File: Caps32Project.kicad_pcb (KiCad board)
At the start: 2 copper layers, 20.8 x 24.6 mm, 53 parts, among them J1 USB_C_Receptacle_USB2.0_16P, J2 SH1.0, Q1 AO3401A, SW1 Reset, SW2 Boot, SW3 SW_SPDT, U1 MPU-6050, U2 AP2112K-3.3, U3 MCP73831-2-OT, U4 ESP32-S2, Y1 40MHz

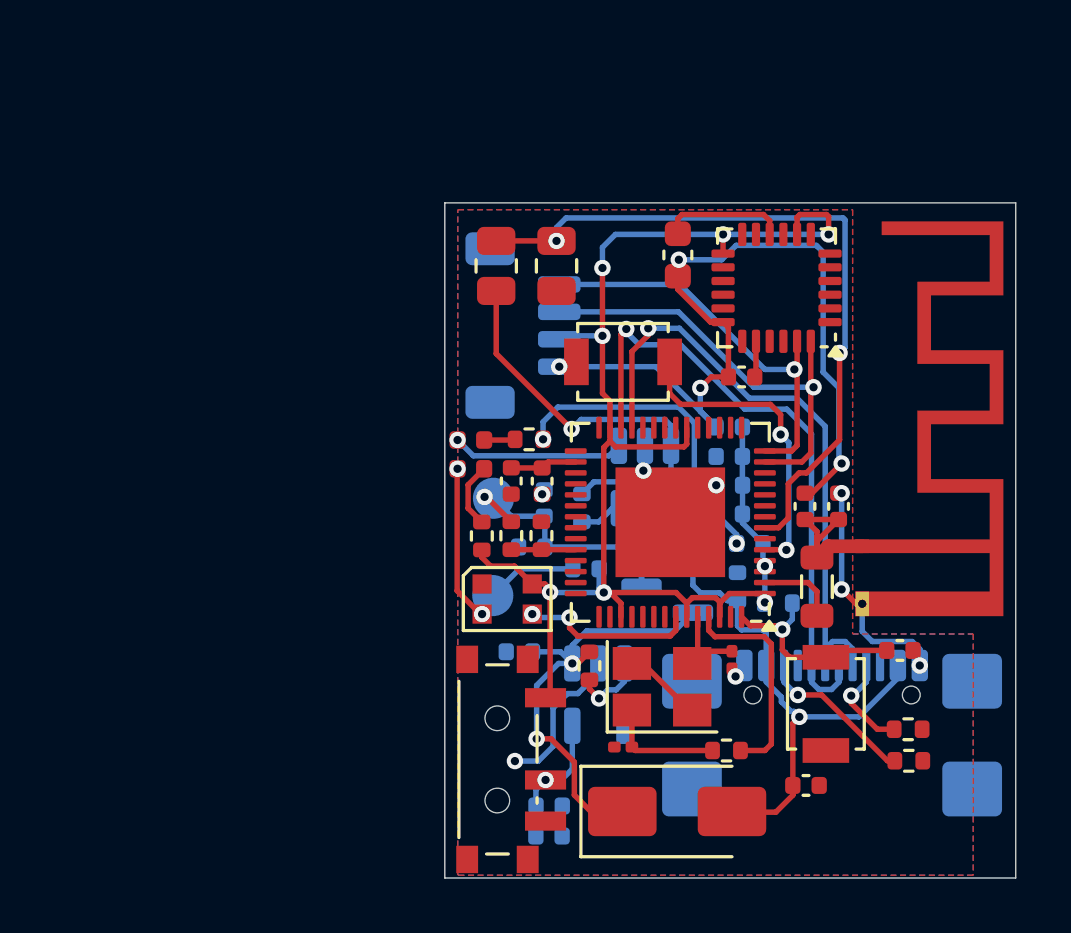
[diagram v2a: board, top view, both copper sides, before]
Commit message: Update Board
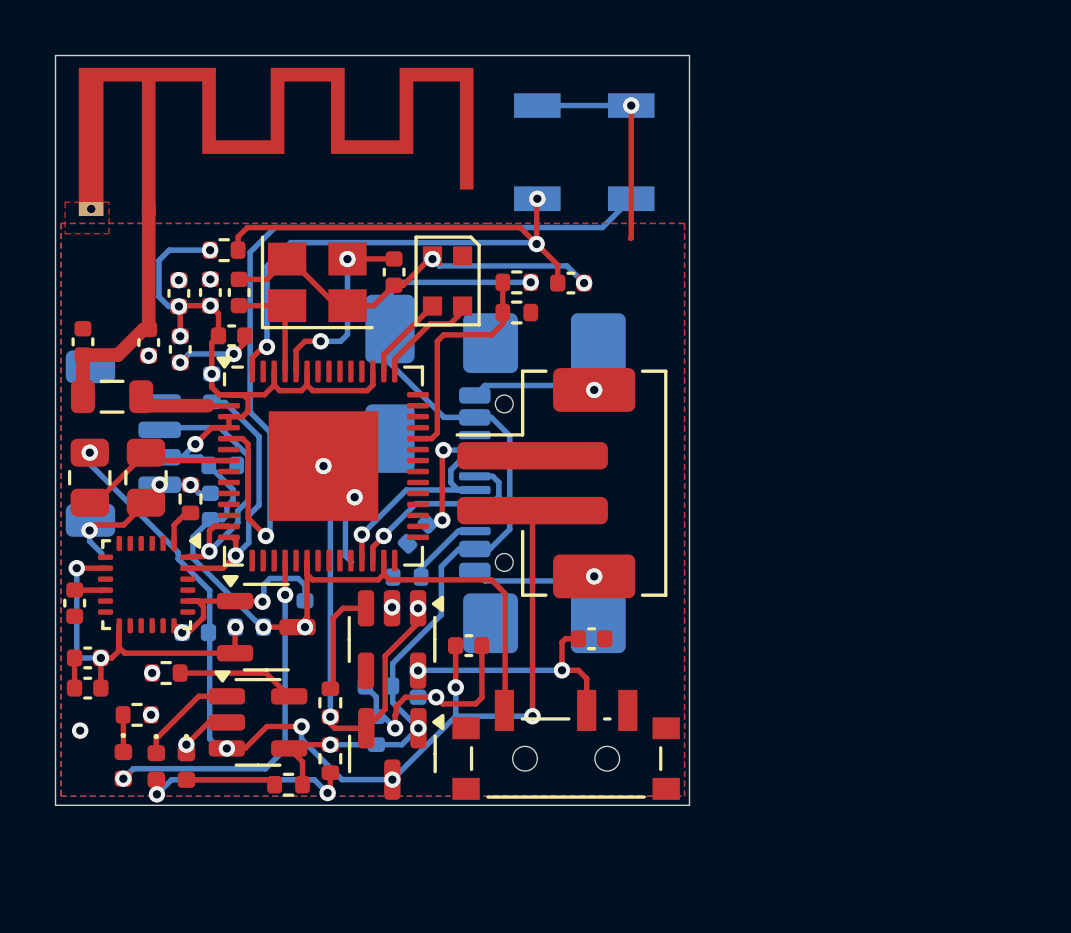
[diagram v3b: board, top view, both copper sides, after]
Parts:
- removed TP1, TP2: TestPoint, TestPoint:TestPoint_Pad_D1.5mm
- added C22: 0.1uF, Capacitor_SMD:C_0402_1005Metric, F.Cu at (112.4, 49.1)
- added C23: 1uF, Capacitor_SMD:C_0402_1005Metric, F.Cu at (110.0, 49.0)
- added D5: WS2812B, LED_SMD:LED_WS2812B-2020_PLCC4_2.0x2.0mm, F.Cu at (123.3, 46.8)
- added J3: USB_C_Receptacle_USB2.0_16P, Connector_USB:USB_C_Receptacle_GCT_USB4110, B.Cu at (128.0, 54.2)
- added R14: 2K, Resistor_SMD:R_0402_1005Metric, F.Cu at (125.8, 48.0)
- added R15: 2K, Resistor_SMD:R_0402_1005Metric, F.Cu at (113.1, 61.1)
- added R16: 5.1K, Resistor_SMD:R_0402_1005Metric, B.Cu at (122.2, 56.0)
- added R17: 5.1K, Resistor_SMD:R_0402_1005Metric, B.Cu at (121.8, 57.6)
- added U5: ESP32-S2, Package_DFN_QFN:QFN-56-1EP_7x7mm_P0.4mm_EP4x4mm, F.Cu at (118.8, 53.6)
- AE1: footprint RF_Antenna:Texas_SWRA117D_2.4GHz_Left -> RF_Antenna:Texas_SWRA117D_2.4GHz_Right
- C1: value 1.0uF -> 1uF; moved to F.Cu
- C10: value 15pF -> 0.1uF; footprint Capacitor_SMD:C_0201_0603Metric -> Capacitor_SMD:C_0402_1005Metric; moved to B.Cu
- C11: value 4.7uF -> 1.0uF; moved to F.Cu
- C12: value 1.0uF -> 0.1uF
- C13, C19: value 0.1uF -> 10uF
- C14: value 1uF -> 0.1uF; moved to F.Cu
- C16, C18, Q1, R8, R9, U2: moved to F.Cu
- C17: value 0.1uF -> 1uF; moved to F.Cu
- C2: value 0.1uF -> 1uF
- C20, C21: value 1uF -> 15pF
- C3: value 1uF -> 1.0uF; moved to B.Cu
- C5: value 1.0uF -> 0.1uF; moved to F.Cu
- C6: value 2.2nF -> 1uF; footprint Capacitor_SMD:C_0603_1608Metric -> Capacitor_SMD:C_0402_1005Metric
- C7, D2: moved to B.Cu
- C8: value 4.7uF -> 1uF; moved to B.Cu
- C9: value 15pF -> 1.0uF; footprint Capacitor_SMD:C_0201_0603Metric -> Capacitor_SMD:C_0402_1005Metric; moved to B.Cu
- D1: value LED -> RED
- D3: value LED -> BLUE
- D4: value WS2812B-2020 -> Orange; footprint LED_SMD:LED_WS2812B-2020_PLCC4_2.0x2.0mm -> LED_SMD:LED_0402_1005Metric
- J1: value USB_C_Receptacle_USB2.0_16P -> Conn_01x02_MountingPin; footprint Connector_USB:USB_C_Receptacle_GCT_USB4110 -> Connector_JST:JST_PH_B2B-PH-SM4-TB_1x02-1MP_P2.00mm_Vertical; moved to F.Cu
- R1: value 1K -> 10K; moved to B.Cu
- R12: value 3K3 -> NC
- R13: value 2K -> 3K3
- R2: value 10K -> 2K; moved to F.Cu
- R3: value 100K -> NC; moved to B.Cu
- R4: value 0 -> 2K
- R5: value 1K -> 100K
- R6, R7: value 5.1K -> 10K; moved to B.Cu
- SW1: value Reset -> SW_SPDT; footprint Button_Switch_SMD:SW_SPST_B3U-1000P -> Button_Switch_SMD:SW_SPDT_PCM12
- SW2: value Boot -> Reset; moved to B.Cu
- SW3: value SW_SPDT -> Boot; footprint Button_Switch_SMD:SW_SPDT_PCM12 -> Button_Switch_SMD:SW_SPST_B3U-1000P; moved to B.Cu
- U1: value MPU-6050 -> XC6206P182MR; footprint Sensor_Motion:InvenSense_QFN-24_4x4mm_P0.5mm -> Package_TO_SOT_SMD:SOT-23-3
- U3: value MCP73831-2-OT -> MPU-9250; footprint Package_TO_SOT_SMD:SOT-23-5 -> Sensor_Motion:InvenSense_QFN-24_3x3mm_P0.4mm; moved to F.Cu
- U4: value ESP32-S2 -> MCP73831-2-OT; footprint Package_DFN_QFN:QFN-56-1EP_7x7mm_P0.4mm_EP4x4mm -> Package_TO_SOT_SMD:SOT-23-5
- moved C8 29.1 mm to (113.5, 47.3), turned to 90 degrees
- moved R7 28.8 mm to (114.7, 50.7), turned to 90 degrees
- moved AE1 28.8 mm to (112.4, 44.2), turned to 0 degrees
- moved C2 27.9 mm to (110.2, 60.6), turned to 180 degrees
- moved R6 26.8 mm to (115.1, 53.5)
- moved L1 26.6 mm to (111.1, 51.0), turned to 180 degrees
- moved C17 25.3 mm to (110.2, 61.7)
- moved R9 24.0 mm to (115.2, 45.7)
- moved C5 23.1 mm to (113.5, 47.3), turned to 90 degrees
- moved C21 23.0 mm to (121.4, 46.5), turned to 90 degrees
- moved SW3 22.6 mm to (130.0, 42.1)
- moved R2 22.4 mm to (112.0, 62.6), turned to 0 degrees
- moved U1 22.4 mm to (116.7, 59.5), turned to 0 degrees
- moved C15 21.9 mm to (113.6, 49.3), turned to -90 degrees
- moved C14 20.6 mm to (113.6, 49.3), turned to -90 degrees
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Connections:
- C1 pad 1: Net-(D2-K) -> +3V3
- C10 pad 1: GND -> +3V3
- C10 pad 2: XTAL_N -> GND
- C11 pad 1: +BATT -> Net-(SW1-B)
- C12 pad 1: +BATT -> +3V3
- C13 pad 1: +3V3 -> VBUS
- C16 pad 1: +3V3 -> RESET
- C17 pad 1: +3V3 -> +1V8
- C18 pad 1: +3V3 -> Net-(U3-REGOUT)
- C19 pad 1: VDD_SPI -> +BATT
- C2 pad 1: GND -> +1V8
- C2 pad 2: Net-(AE1-FEED) -> GND
- C20 pad 1: VDD_SPI -> GND
- C20 pad 2: GND -> XTAL_P
- C21 pad 1: RESET -> GND
- C21 pad 2: GND -> XTAL_N
- C3 pad 1: GND -> Net-(D2-K)
- C3 pad 2: Net-(AE1-FEED) -> GND
- C4 pad 1: Net-(SW3-B) -> +BATT
- C5 pad 1: Net-(SW3-B) -> +3V3
- C6 pad 1: GND -> +3V3
- C6 pad 2: Net-(U1-REGOUT) -> GND
- C7 pad 1: Net-(U1-CPOUT) -> +3V3
- C8 pad 1: VBUS -> +3V3
- C9 pad 1: GND -> Net-(SW1-B)
- C9 pad 2: Net-(C9-Pad2) -> GND
- D1 pad 1: GND -> Net-(D1-K)
- D1 pad 2: Net-(D1-A) -> IO13
- D3 pad 1: Net-(D3-K) -> GND
- D4 pad 1: unconnected-(D4-DOUT-Pad1) -> Net-(D4-K)
- D4 pad 2: GND -> Net-(D4-A)
- R1 pad 1: +3V3 -> VBUS
- R1 pad 2: Net-(D1-A) -> GND
- R12 pad 1: +BATT -> Net-(U3-RESV_VDDIO)
- R12 pad 2: IO34 -> GND
- R13 pad 1: IO34 -> VBUS
- R13 pad 2: GND -> IO34
- R2 pad 1: VBUS -> Net-(D1-K)
- R3 pad 1: Net-(D2-K) -> +1V8
- R3 pad 2: Net-(U2-EN) -> +3V3
- R4 pad 1: Net-(C9-Pad2) -> VBUS
- R4 pad 2: XTAL_P -> Net-(D3-A)
- R5 pad 1: VBUS -> Net-(D2-K)
- R5 pad 2: Net-(D3-A) -> Net-(U2-EN)
- R6 pad 1: Net-(J1-CC1) -> +3V3
- R6 pad 2: GND -> SDA
- R7 pad 1: Net-(J1-CC2) -> SCL
- R7 pad 2: GND -> +3V3
- R8 pad 1: Net-(U3-PROG) -> VBUS
- R8 pad 2: GND -> Net-(D4-A)
- SW1 pad 1: GND -> +3V3
- SW1 pad 2: RESET -> Net-(SW1-B)
- SW2 pad 2: BOOT -> RESET
- SW3 pad 1: +3V3 -> GND
- SW3 pad 2: Net-(SW3-B) -> BOOT
- U1 pad 1: unconnected-(U1-CLKIN-Pad1) -> GND
- U1 pad 2: unconnected-(U1-NC-Pad2) -> +1V8
- U1 pad 3: unconnected-(U1-NC-Pad3) -> +3V3
- U2 pad 5: Net-(SW3-B) -> Net-(SW1-B)
- U3 pad 1: Net-(D3-K) -> Net-(U3-RESV_VDDIO)
- U3 pad 2: GND -> (no net)
- U3 pad 3: +BATT -> (no net)
- U3 pad 4: VBUS -> (no net)
- U3 pad 5: Net-(U3-PROG) -> (no net)
- U4 pad 1: +3V3 -> Net-(D4-K)
- U4 pad 2: LNA -> GND
- U4 pad 3: +3V3 -> +BATT
- U4 pad 4: +3V3 -> VBUS
- U4 pad 5: BOOT -> Net-(U4-PROG)
- Y1 pad 1: Net-(C9-Pad2) -> XTAL_P
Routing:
- net RESET: track 7.56 -> 29.6 mm, vias 1 -> 3
- net IO2: track 26.3 -> 5.95 mm, vias 2 -> 0
- net BOOT: track 11.4 -> 29.8 mm, vias 2 -> 1
- net USB_P: track 23.0 -> 7.34 mm
- net USB_N: track 23.0 -> 8.18 mm
- net +1V8: track 0.00 -> 14.0 mm, vias 0 -> 3
- net IO13: track 0.00 -> 13.2 mm, vias 0 -> 2
- net +BATT: track 26.0 -> 36.6 mm, vias 2 -> 6
- net Net-(SW1-B): track 0.00 -> 9.12 mm, vias 0 -> 2
- net Net-(D4-A): track 0.00 -> 7.97 mm, vias 0 -> 2
- net +3V3: track 56.6 -> 50.0 mm
- net RGB: track 6.37 -> 0.00 mm, vias 2 -> 0
- net Net-(D3-K): track 6.27 -> 0.00 mm, vias 1 -> 0
- net IO34: track 2.35 -> 8.30 mm
- net Net-(J1-CC2): track 5.84 -> 0.00 mm, vias 1 -> 0
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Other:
- board size 20.8 x 24.6 mm -> 23.1 x 27.4 mm

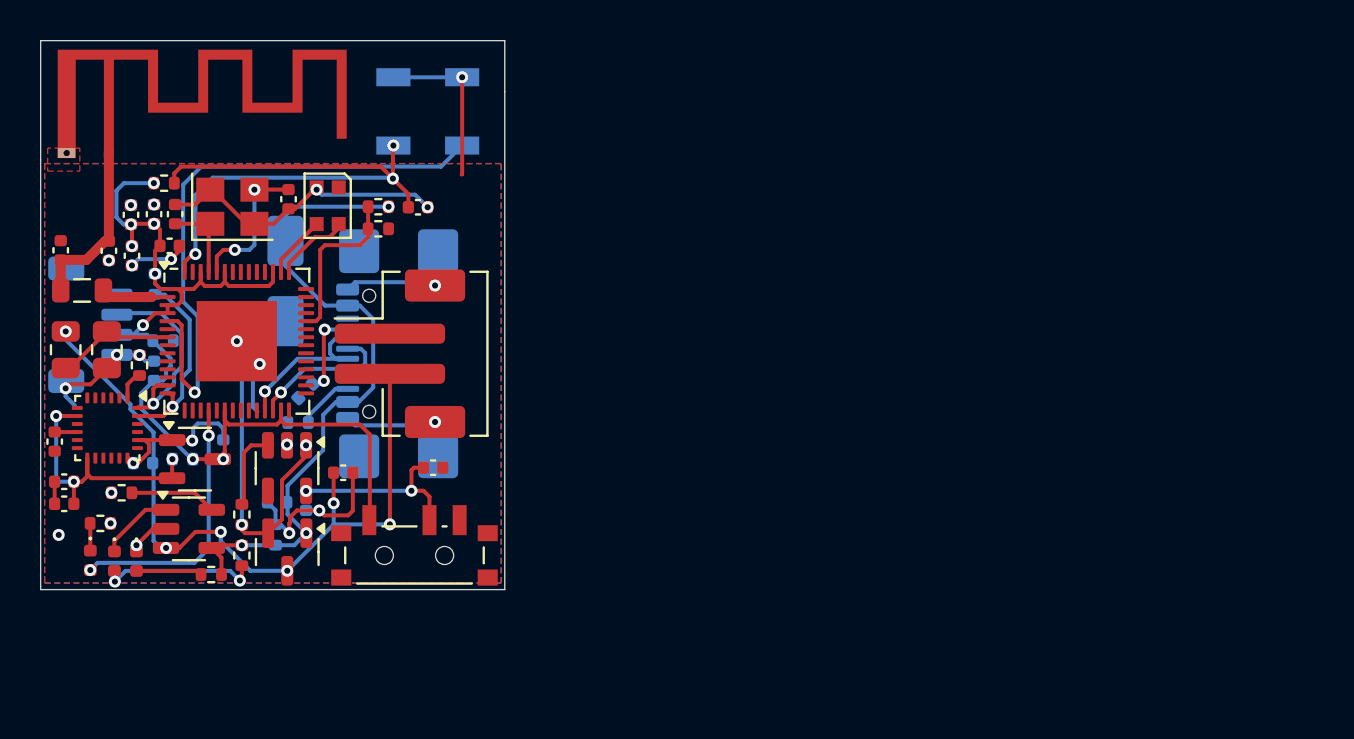
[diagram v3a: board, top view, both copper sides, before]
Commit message: Update Board
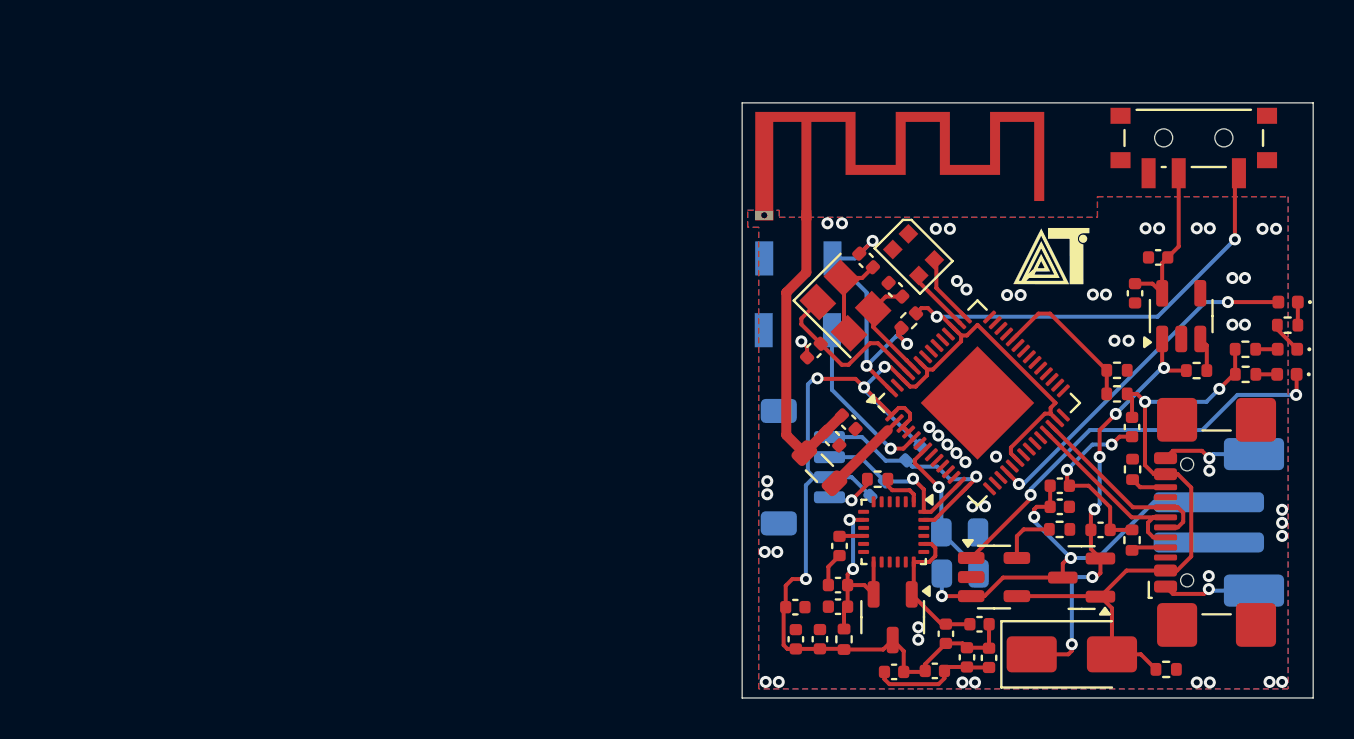
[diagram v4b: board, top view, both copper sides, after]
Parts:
- added G***: LOGO, LOGO, F.Cu at (159.3, 49.3)
- C10, C12, C13, C15, C3, C4, C7, C8, C9, D2, J3, R1, R16, R17, R3: moved to F.Cu
- J1, R10, R11: moved to B.Cu
- moved D1 61.0 mm to (171.2, 51.6), turned to 180 degrees
- moved R2 60.0 mm to (171.2, 52.8), turned to 180 degrees
- moved D4 59.2 mm to (171.1, 55.2), turned to 180 degrees
- moved D3 58.3 mm to (171.1, 54.0), turned to 180 degrees
- moved R4 52.7 mm to (169.0, 54.0), turned to 0 degrees
- moved R8 50.8 mm to (169.1, 55.2), turned to 0 degrees
- moved R5 48.1 mm to (166.6, 55.0), turned to 0 degrees
- moved C14 47.2 mm to (156.3, 69.3)
- moved C8 46.9 mm to (155.8, 67.7), turned to 180 degrees
- moved R15 46.8 mm to (159.8, 63.0), turned to 0 degrees
- moved C7 46.1 mm to (155.2, 69.3), turned to -90 degrees
- moved R10 45.9 mm to (154.8, 65.2), turned to 0 degrees
- moved C4 45.7 mm to (159.8, 61.8), turned to 0 degrees
- moved U2 45.2 mm to (165.8, 52.3), turned to 90 degrees
- moved C15 45.0 mm to (153.6, 70.0), turned to 0 degrees
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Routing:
- net +3V3: track 50.0 -> 84.1 mm, vias 8 -> 6
- net BOOT: track 29.8 -> 8.52 mm
- net GND: track 64.3 -> 44.0 mm, vias 24 -> 55
- net Net-(D4-K): track 3.74 -> 20.9 mm, vias 0 -> 2
- net +BATT: track 36.6 -> 21.8 mm, vias 6 -> 3
- net RESET: track 29.6 -> 14.9 mm
- net Net-(D4-A): track 7.97 -> 1.06 mm, vias 2 -> 0
- net Net-(AE1-FEED): track 8.70 -> 15.3 mm
- net XTAL_P: track 4.18 -> 8.71 mm
- net +1V8: track 14.0 -> 9.50 mm, vias 3 -> 2
- net IO13: track 13.2 -> 17.5 mm
- net Net-(D2-K): track 17.8 -> 21.7 mm, vias 2 -> 6
- net Net-(J3-CC1): track 4.34 -> 1.73 mm, vias 2 -> 0
- net USB_P: track 7.34 -> 9.77 mm, vias 1 -> 0
- net Net-(U2-EN): track 3.97 -> 1.71 mm
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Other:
- board size 23.1 x 27.4 mm -> 28.5 x 29.6 mm
- board text added: "+"
- board text added: "-"
- board text added: "Boot"
- board text added: "Reset"
